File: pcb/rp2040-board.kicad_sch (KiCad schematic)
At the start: 61 parts, among them J1 DMX, J2 GPIO, J3 ELRS, J4 OLED, J5 SWD, J6 USB_C_Receptacle_USB2.0_16P, J7 AUDIO, SW1 TS-1187A-B-A-B, SW2 RotaryEncoder_Switch, SW3 TS-1187A-B-A-B, U1 W25Q128JVS, U2 SP485EEN-L/TR, U3 RP2040, U4 AMS1117-3.3, U5 OP07CDR, Y1 12MHz

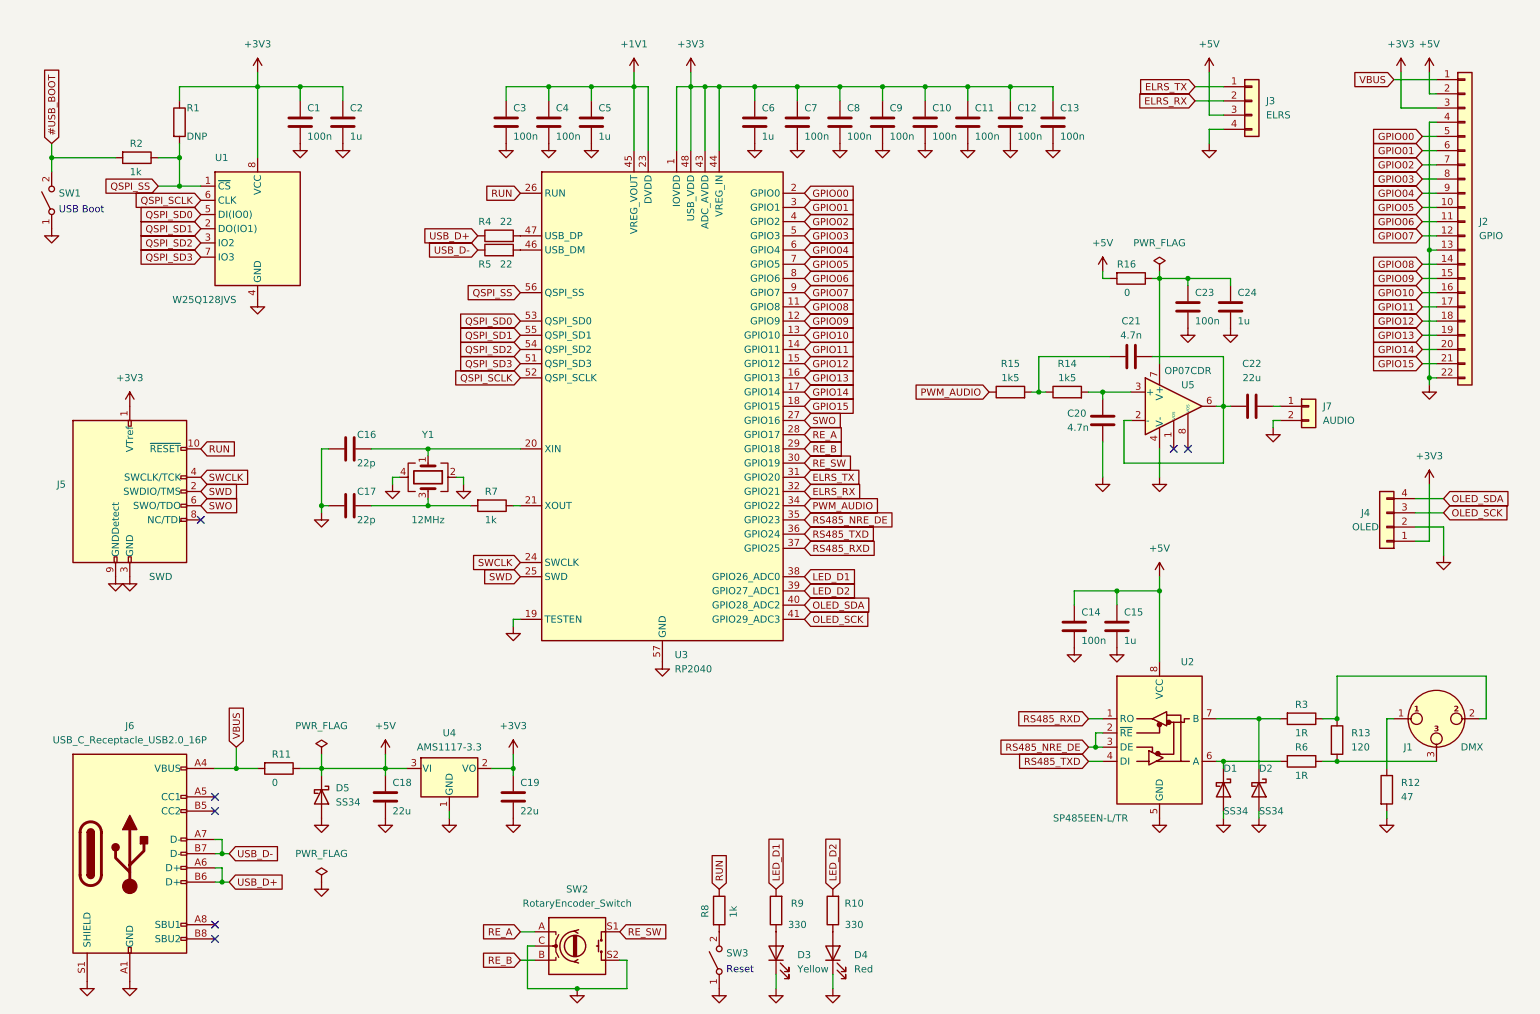
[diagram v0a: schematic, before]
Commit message: WIP on the second PCB, also resaved with kicad 9
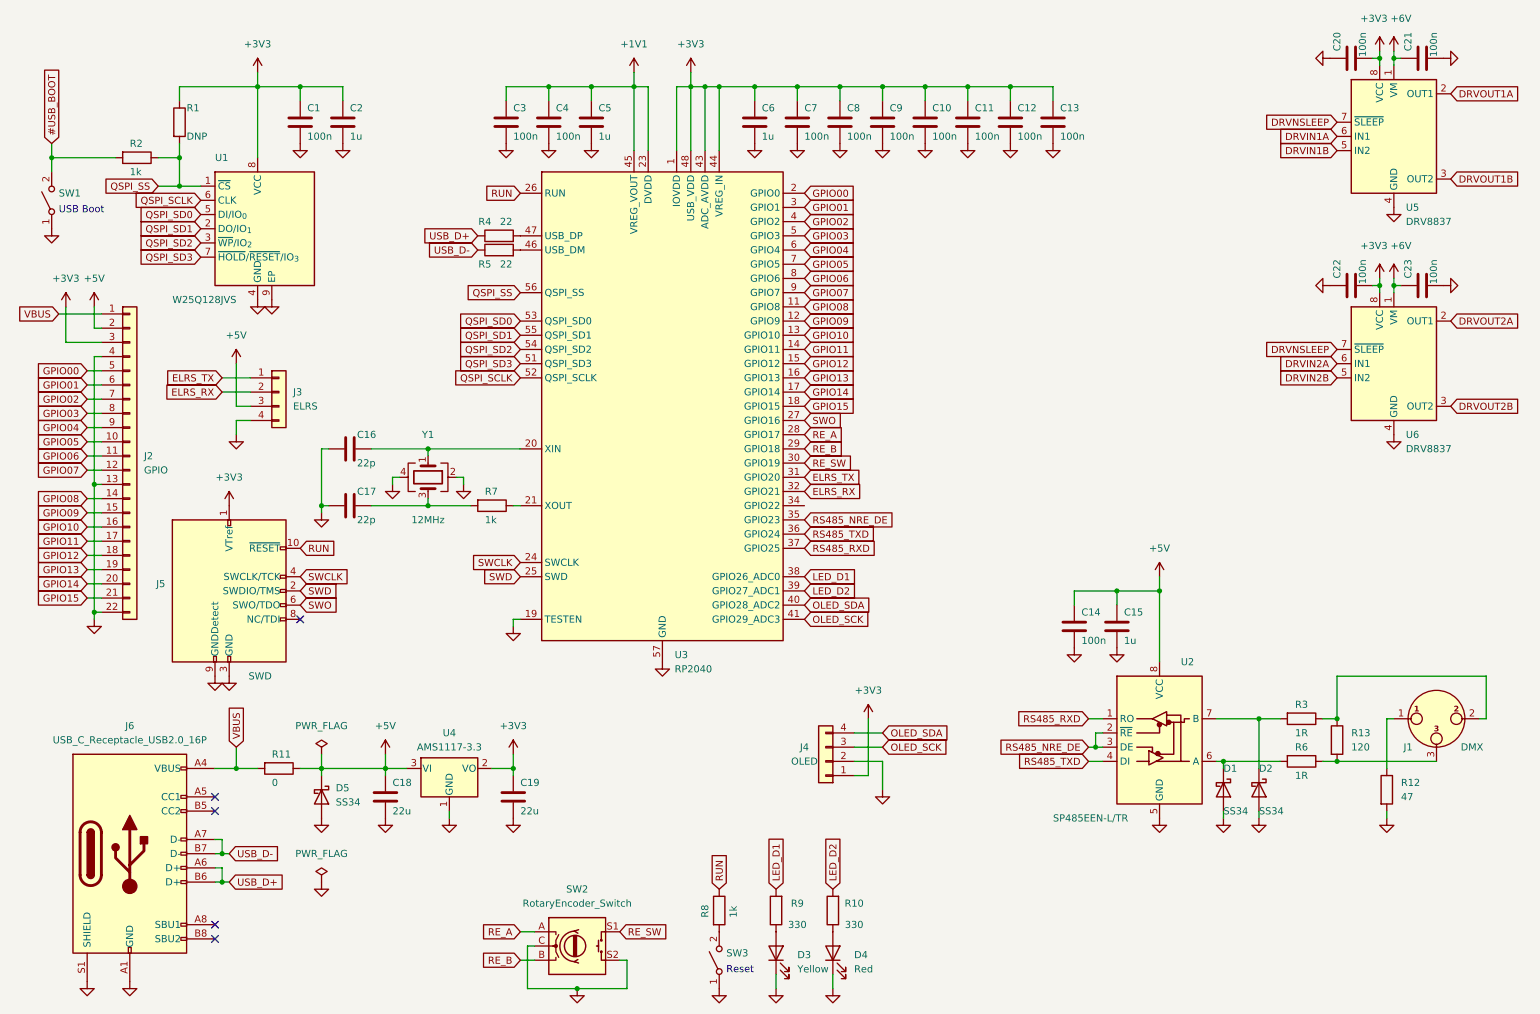
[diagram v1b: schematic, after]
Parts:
- removed C24: 1u, Capacitor_SMD:C_0402_1005Metric, symbol Device:C
- removed J7: AUDIO, Connector_PinHeader_2.54mm:PinHeader_1x02_P2.54mm_Vertical, symbol Connector_Generic:Conn_01x02
- removed R14, R15: 1k5, Resistor_SMD:R_0402_1005Metric, symbol Device:R
- removed R16: 0, Resistor_SMD:R_0603_1608Metric, symbol Device:R
- removed U5: OP07CDR, Package_SO:SOIC-8_3.9x4.9mm_P1.27mm, symbol Amplifier_Operational:OP07
- added U5, U6: DRV8837, Package_SON:WSON-8-1EP_2x2mm_P0.5mm_EP0.9x1.6mm, symbol Driver_Motor:DRV8837
- C20, C21: value 4.7n -> 100n; LCSC Part C1538 -> C1525
- C22: value 22u -> 100n; footprint Capacitor_SMD:C_0805_2012Metric -> Capacitor_SMD:C_0402_1005Metric; LCSC Part C45783 -> C1525
- U1: footprint Package_SO:SOIC-8_5.23x5.23mm_P1.27mm -> Package_SON:WSON-8-1EP_6x5mm_P1.27mm_EP3.4x4.3mm; symbol Memory_Flash:W25Q128JVS -> Memory_Flash:W25Q32JVZP; LCSC Part C97521 -> C571260
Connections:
- net +3V3: now also C20.2, C22.2, U5.8 (VCC), U6.8 (VCC)
- net GND: now also C20.1, C21.2, C22.1, U1.9 (EP), U5.4 (GND), U5.9 (GND), U6.4 (GND), U6.9 (GND); no longer C20.2
- net +6V: now reaches C21.1
- net +6V: now also C23.1, U5.1 (VM), U6.1 (VM)
- net PWM_AUDIO: no longer names the net of U3.34 (GPIO22)
- new net DRVIN1A: U5.6 (IN1)
- new net DRVIN1B: U5.5 (IN2)
- new net DRVIN2A: U6.6 (IN1)
- new net DRVIN2B: U6.5 (IN2)
- new net DRVNSLEEP: U5.7 (~{SLEEP}), U6.7 (~{SLEEP})
- new net DRVOUT1A: U5.2 (OUT1)
- new net DRVOUT1B: U5.3 (OUT2)
- new net DRVOUT2A: U6.2 (OUT1)
- new net DRVOUT2B: U6.3 (OUT2)
- no-connect marks 7 -> 5
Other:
- moved on the sheet: J2, J3, J4, J5
